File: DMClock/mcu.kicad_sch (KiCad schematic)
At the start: 2 parts, among them U1 PIC16F18346-P, U2 DS3231SN_

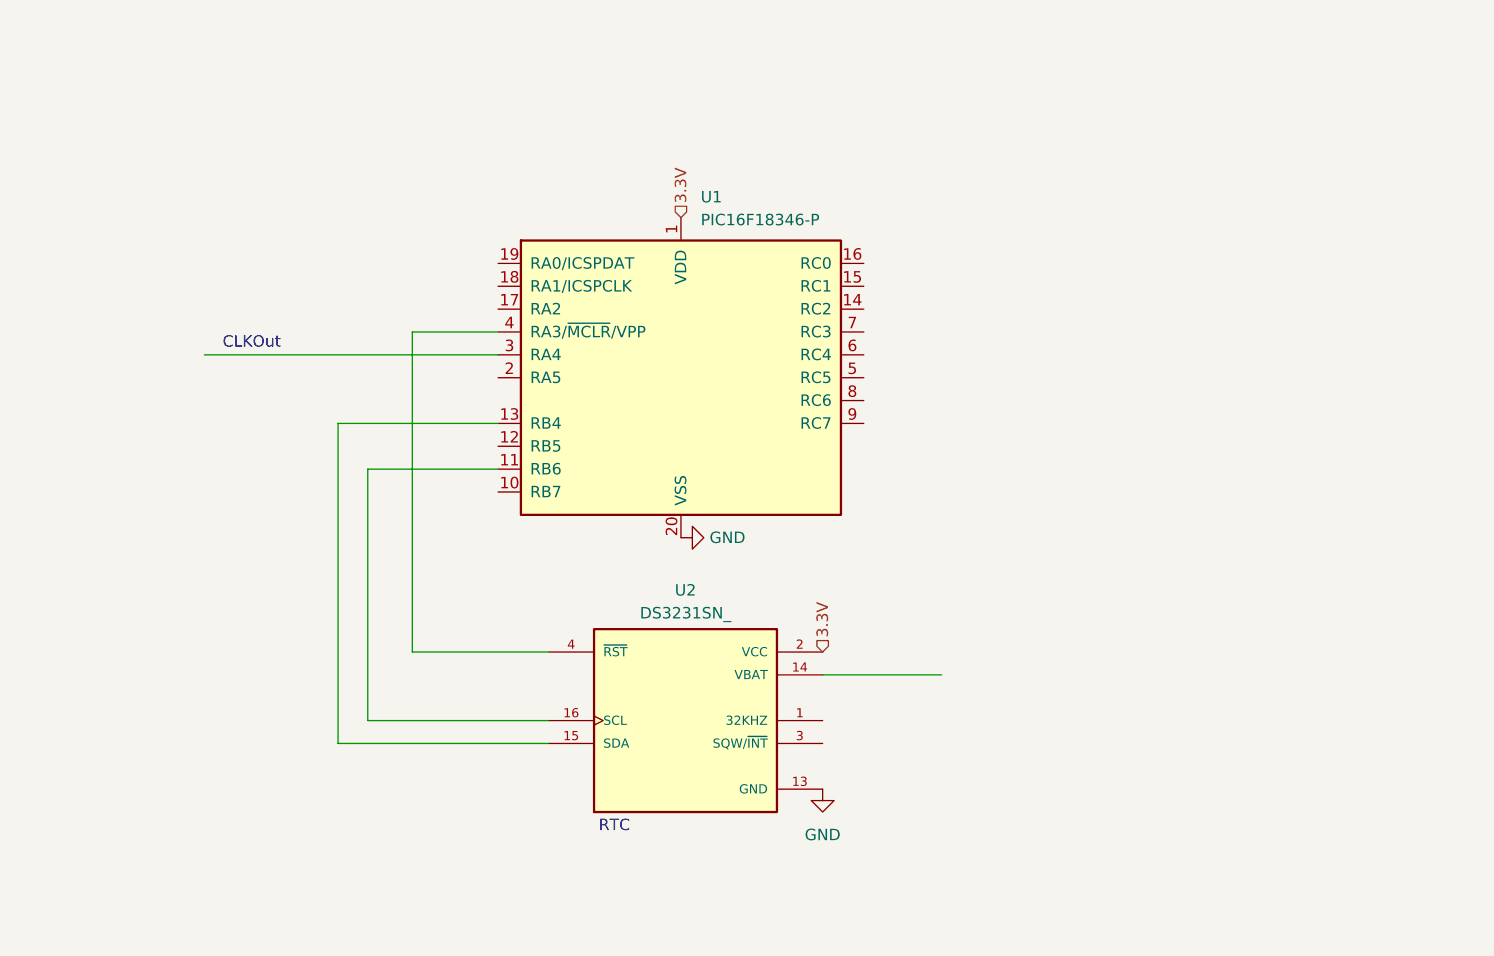
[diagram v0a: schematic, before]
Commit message: need to work on hvps logic converter
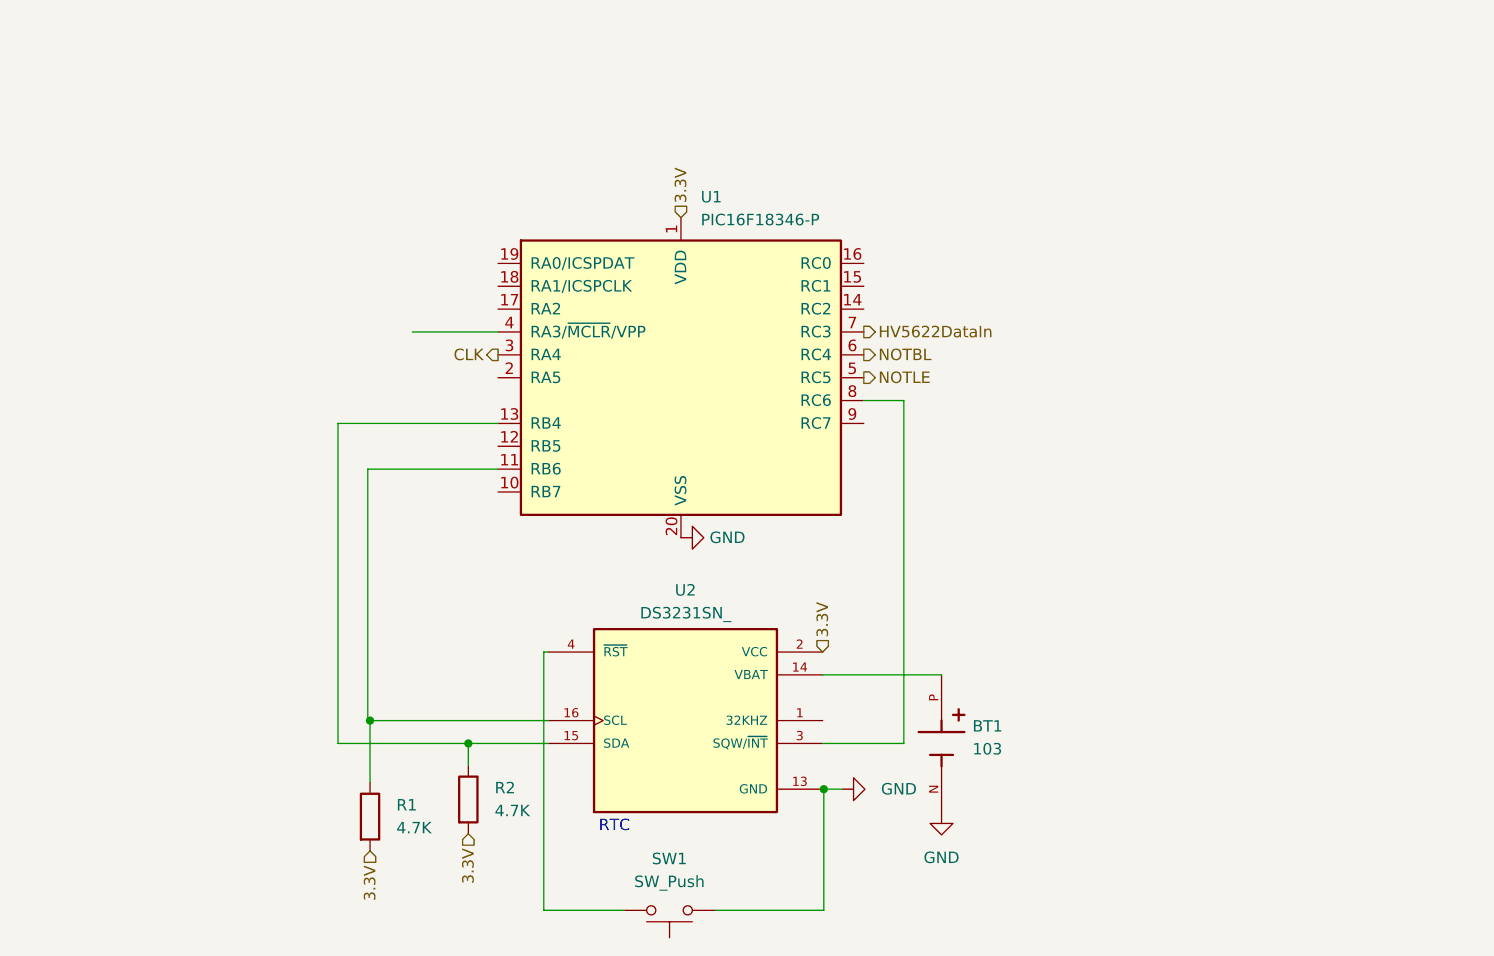
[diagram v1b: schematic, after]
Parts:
- added BT1: 103, Footprints:BAT_103, symbol 103:103
- added R1, R2: 4.7K, Resistor_THT:R_Axial_DIN0204_L3.6mm_D1.6mm_P2.54mm_Vertical, symbol Device:R
- added SW1: SW_Push, symbol Switch:SW_Push
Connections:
- net 3.3V: now also R1.2, R2.2
- net GND: now also BT1.N, SW1.1
- net at U2.14 (VBAT): now also BT1.P
- net at U1.13 (RB4), U2.15 (SDA): now also R2.1
- net at U1.11 (RB6), U2.16 (SCL): now also R1.1
- net at U2.3 (SQW/~{INT}): now also U1.8 (RC6)
- net at U2.4 (~{RST}): now also SW1.2; no longer U1.4 (RA3/~{MCLR}/VPP)
- net CLK: now reaches U1.3 (RA4)
- net NOTLE: now reaches U1.5 (RC5)
- net NOTBL: now reaches U1.6 (RC4)
- net HV5622DataIn: now reaches U1.7 (RC3)
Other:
- note removed: "CLKOut"

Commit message: just need to finish pcb
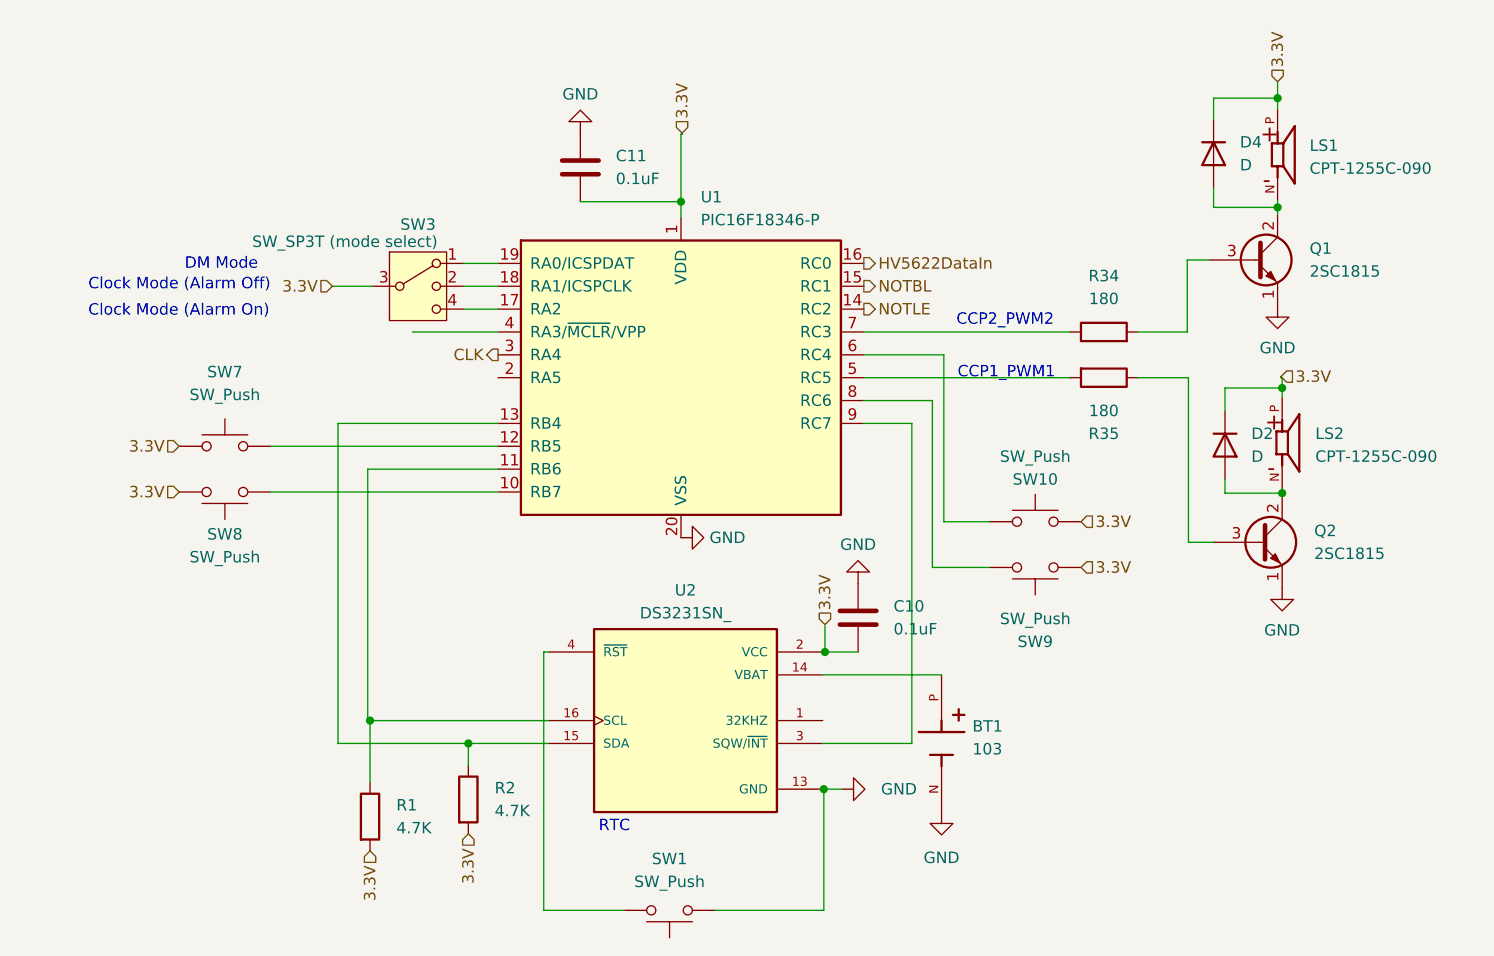
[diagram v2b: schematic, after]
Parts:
- added C10, C11: 0.1uF, Capacitor_SMD:C_0805_2012Metric, symbol Device:C
- added D2, D4: D, Diode_THT:D_A-405_P2.54mm_Vertical_AnodeUp, symbol Device:D
- added LS1, LS2: CPT-1255C-090, Footprints:CUI_CPT-1255C-090, symbol CPT-1255C-090:CPT-1255C-090
- added Q1, Q2: 2SC1815, Package_TO_SOT_THT:TO-92_Inline, symbol Transistor_BJT:2SC1815
- added R34, R35: 180, Resistor_THT:R_Axial_DIN0204_L3.6mm_D1.6mm_P2.54mm_Vertical, symbol Device:R
- added SW10, SW7, SW8, SW9: SW_Push, Connector_PinHeader_2.54mm:PinHeader_1x02_P2.54mm_Vertical, symbol Switch:SW_Push
- added SW3: SW_SP3T (mode select), Footprints:OS102011MS8QP1, symbol Switch:SW_SP3T
- SW1: footprint (none) -> Connector_PinHeader_2.54mm:PinHeader_1x02_P2.54mm_Vertical
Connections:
- net 3.3V: now also C11.1, D2.1 (K), D4.1 (K), LS1.P, LS2.P, SW10.2, SW3.3, SW7.1, SW8.2, SW9.1; no longer U2.2 (VCC)
- net GND: now also C10.2, C11.2, Q1.1 (E), Q2.1 (E)
- net HV5622DataIn: now also U1.16 (RC0); no longer U1.7 (RC3)
- net NOTBL: now also U1.15 (RC1); no longer U1.6 (RC4)
- net NOTLE: now also U1.14 (RC2); no longer U1.5 (RC5)
- net at U2.3 (SQW/~{INT}): now also U1.9 (RC7); no longer U1.8 (RC6)
- net at U1.10 (RB7): now also SW8.1
- net at U1.12 (RB5): now also SW7.2
- net at U1.17 (RA2): now also SW3.4
- net at U1.18 (RA1/ICSPCLK): now also SW3.2
- net at U1.19 (RA0/ICSPDAT): now also SW3.1
- new net: D2.2 (A), LS2.N, Q2.2 (C)
- new net: SW10.1, U1.6 (RC4)
- new net: C10.1, U2.2 (VCC)
- new net: Q2.3 (B), R35.1
- new net: D4.2 (A), LS1.N, Q1.2 (C)
- new net: Q1.3 (B), R34.2
- new net: R35.2, U1.5 (RC5)
- new net: SW9.2, U1.8 (RC6)
- new net: R34.1, U1.7 (RC3)
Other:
- note added: "CCP1_PWM1"
- note added: "CCP2_PWM2"
- note added: "Clock Mode (Alarm Off)"
- note added: "Clock Mode (Alarm On)"
- note added: "DM Mode"
